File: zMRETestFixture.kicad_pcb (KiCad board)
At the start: 2 copper layers, 106.7 x 124.5 mm, 120 parts, among them J1 Conn_01x01, J2 Conn_01x01, J3 Conn_01x01_Female, J4 Conn_01x01_Female, J5 Conn_01x01, J6 Conn_01x01, J7 Conn_01x01, J8 Conn_01x01, J9 Conn_02x05_Counter_Clockwise, SW1 SW_Push, SW2 SW_Push, U1 molex_48pin_MRE

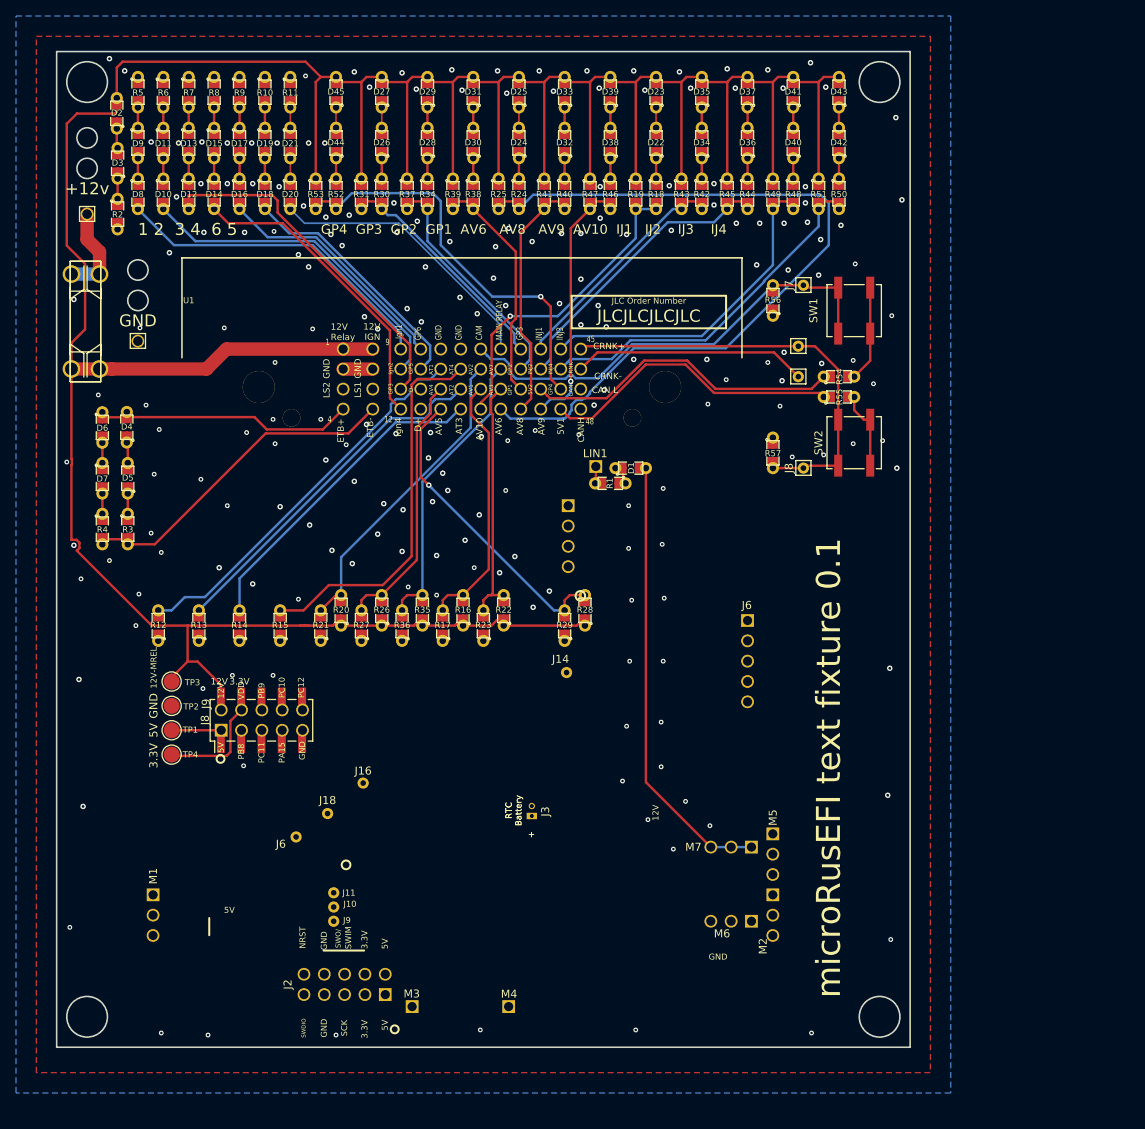
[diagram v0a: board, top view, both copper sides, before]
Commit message: DRAFT`
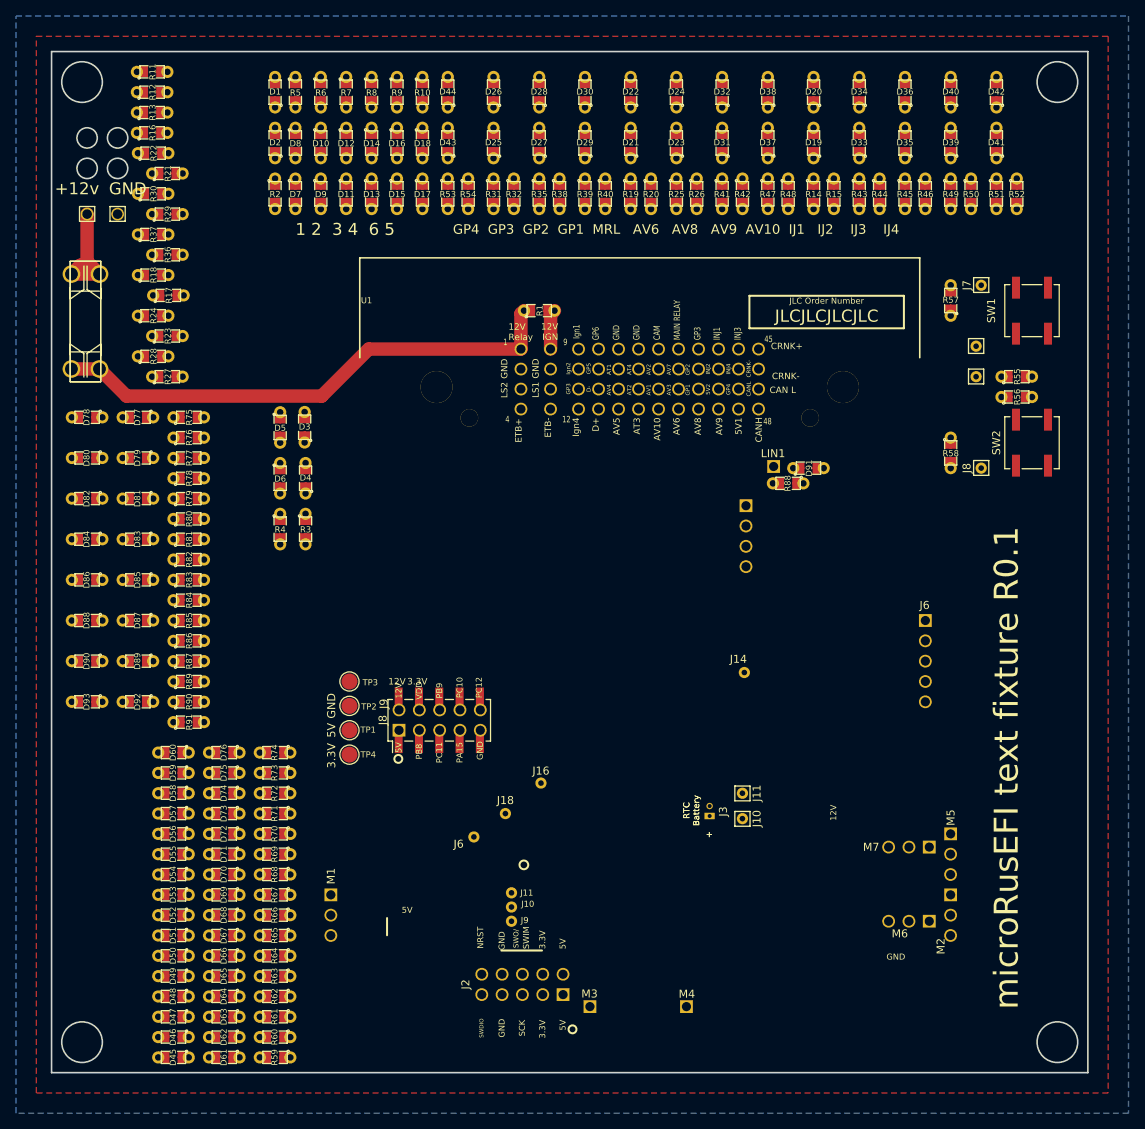
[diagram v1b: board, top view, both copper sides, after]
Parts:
- removed R34: 1k, rusefi_lib:SM0805_jumper
- added D46: 1N4148WS, rusefi_lib:SM0805_jumper, F.Cu at (45.1, 150.5)
- added D47: 1N4148WS, rusefi_lib:SM0805_jumper, F.Cu at (45.1, 148.0)
- added D48: 1N4148WS, rusefi_lib:SM0805_jumper, F.Cu at (45.1, 145.4)
- added D49: 1N4148WS, rusefi_lib:SM0805_jumper, F.Cu at (45.1, 142.9)
- added D50: 1N4148WS, rusefi_lib:SM0805_jumper, F.Cu at (45.1, 140.3)
- added D51: 1N4148WS, rusefi_lib:SM0805_jumper, F.Cu at (45.1, 137.8)
- added D52: 1N4148WS, rusefi_lib:SM0805_jumper, F.Cu at (45.1, 135.3)
- added D53: 1N4148WS, rusefi_lib:SM0805_jumper, F.Cu at (45.1, 132.7)
- added D54: 1N4148WS, rusefi_lib:SM0805_jumper, F.Cu at (45.1, 130.2)
- added D55: 1N4148WS, rusefi_lib:SM0805_jumper, F.Cu at (45.1, 127.6)
- added D56: 1N4148WS, rusefi_lib:SM0805_jumper, F.Cu at (45.1, 125.1)
- added D57: 1N4148WS, rusefi_lib:SM0805_jumper, F.Cu at (45.1, 122.6)
- added D58: 1N4148WS, rusefi_lib:SM0805_jumper, F.Cu at (45.1, 120.0)
- added D59: 1N4148WS, rusefi_lib:SM0805_jumper, F.Cu at (45.1, 117.5)
- added D60: 1N4148WS, rusefi_lib:SM0805_jumper, F.Cu at (45.1, 114.9)
- added D61: GRN, rusefi_lib:SM0805_jumper, F.Cu at (51.4, 153.0)
- added D62: GRN, rusefi_lib:SM0805_jumper, F.Cu at (51.4, 150.5)
- added D63: GRN, rusefi_lib:SM0805_jumper, F.Cu at (51.4, 148.0)
- added D64: GRN, rusefi_lib:SM0805_jumper, F.Cu at (51.4, 145.4)
- added D65: GRN, rusefi_lib:SM0805_jumper, F.Cu at (51.4, 142.9)
- added D66: GRN, rusefi_lib:SM0805_jumper, F.Cu at (51.4, 140.3)
- added D67: GRN, rusefi_lib:SM0805_jumper, F.Cu at (51.4, 137.8)
- added D68: GRN, rusefi_lib:SM0805_jumper, F.Cu at (51.4, 135.3)
- added D69: GRN, rusefi_lib:SM0805_jumper, F.Cu at (51.4, 132.7)
- added D70: GRN, rusefi_lib:SM0805_jumper, F.Cu at (51.4, 130.2)
- added D71: GRN, rusefi_lib:SM0805_jumper, F.Cu at (51.4, 127.6)
- added D72: GRN, rusefi_lib:SM0805_jumper, F.Cu at (51.4, 125.1)
- added D73: GRN, rusefi_lib:SM0805_jumper, F.Cu at (51.4, 122.6)
- added D74: GRN, rusefi_lib:SM0805_jumper, F.Cu at (51.4, 120.0)
- added D75: GRN, rusefi_lib:SM0805_jumper, F.Cu at (51.4, 117.5)
- added D76: GRN, rusefi_lib:SM0805_jumper, F.Cu at (51.4, 114.9)
- added D77: RED, rusefi_lib:SM0805_jumper, F.Cu at (40.6, 73.0)
- added D78: 1N4148WS, rusefi_lib:SM0805_jumper, F.Cu at (34.3, 73.0)
- added D79: RED, rusefi_lib:SM0805_jumper, F.Cu at (40.6, 78.1)
- added D80: 1N4148WS, rusefi_lib:SM0805_jumper, F.Cu at (34.3, 78.1)
- added D81: RED, rusefi_lib:SM0805_jumper, F.Cu at (40.6, 83.2)
- added D82: 1N4148WS, rusefi_lib:SM0805_jumper, F.Cu at (34.3, 83.2)
- added D83: RED, rusefi_lib:SM0805_jumper, F.Cu at (40.6, 88.3)
- added D84: 1N4148WS, rusefi_lib:SM0805_jumper, F.Cu at (34.3, 88.3)
- added D85: RED, rusefi_lib:SM0805_jumper, F.Cu at (40.6, 93.3)
- added D86: 1N4148WS, rusefi_lib:SM0805_jumper, F.Cu at (34.3, 93.3)
- added D87: RED, rusefi_lib:SM0805_jumper, F.Cu at (40.6, 98.4)
- added D88: 1N4148WS, rusefi_lib:SM0805_jumper, F.Cu at (34.3, 98.4)
- added D89: RED, rusefi_lib:SM0805_jumper, F.Cu at (40.6, 103.5)
- added D90: 1N4148WS, rusefi_lib:SM0805_jumper, F.Cu at (34.3, 103.5)
- added D91: 1N4148WS, rusefi_lib:SM0805_jumper, F.Cu at (124.5, 79.4)
- added D92: RED, rusefi_lib:SM0805_jumper, F.Cu at (40.6, 108.6)
- added D93: 1N4148WS, rusefi_lib:SM0805_jumper, F.Cu at (34.3, 108.6)
- added J10: Conn_01x01, Connector_Pin:Pin_D0.7mm_L6.5mm_W1.8mm_FlatFork, F.Cu at (116.2, 123.2)
- added J11: Conn_01x01, Connector_Pin:Pin_D0.7mm_L6.5mm_W1.8mm_FlatFork, F.Cu at (116.2, 120.0)
- added R32: 5k, rusefi_lib:SM0805_jumper, F.Cu at (87.6, 45.1)
- added R58: 470k, rusefi_lib:SM0805_jumper, F.Cu at (142.2, 77.5)
- added R59: 1k, rusefi_lib:SM0805_jumper, F.Cu at (57.8, 153.0)
- added R60: 1k, rusefi_lib:SM0805_jumper, F.Cu at (57.8, 150.5)
- added R61: 1k, rusefi_lib:SM0805_jumper, F.Cu at (57.8, 148.0)
- added R62: 1k, rusefi_lib:SM0805_jumper, F.Cu at (57.8, 145.4)
- added R63: 1k, rusefi_lib:SM0805_jumper, F.Cu at (57.8, 142.9)
- added R64: 1k, rusefi_lib:SM0805_jumper, F.Cu at (57.8, 140.3)
- added R65: 1k, rusefi_lib:SM0805_jumper, F.Cu at (57.8, 137.8)
- added R66: 1k, rusefi_lib:SM0805_jumper, F.Cu at (57.8, 135.3)
- added R67: 1k, rusefi_lib:SM0805_jumper, F.Cu at (57.8, 132.7)
- added R68: 1k, rusefi_lib:SM0805_jumper, F.Cu at (57.8, 130.2)
- added R69: 1k, rusefi_lib:SM0805_jumper, F.Cu at (57.8, 127.6)
- added R70: 1k, rusefi_lib:SM0805_jumper, F.Cu at (57.8, 125.1)
- added R71: 1k, rusefi_lib:SM0805_jumper, F.Cu at (57.8, 122.6)
- added R72: 1k, rusefi_lib:SM0805_jumper, F.Cu at (57.8, 120.0)
- added R73: 1k, rusefi_lib:SM0805_jumper, F.Cu at (57.8, 117.5)
- added R74: 1k, rusefi_lib:SM0805_jumper, F.Cu at (57.8, 114.9)
- added R75: 1k, rusefi_lib:SM0805_jumper, F.Cu at (47.0, 73.0)
- added R76: 5k, rusefi_lib:SM0805_jumper, F.Cu at (47.0, 75.6)
- added R77: 1k, rusefi_lib:SM0805_jumper, F.Cu at (47.0, 78.1)
- added R78: 5k, rusefi_lib:SM0805_jumper, F.Cu at (47.0, 80.6)
- added R79: 1k, rusefi_lib:SM0805_jumper, F.Cu at (47.0, 83.2)
- added R80: 5k, rusefi_lib:SM0805_jumper, F.Cu at (47.0, 85.7)
- added R81: 1k, rusefi_lib:SM0805_jumper, F.Cu at (47.0, 88.3)
- added R82: 5k, rusefi_lib:SM0805_jumper, F.Cu at (47.0, 90.8)
- added R83: 1k, rusefi_lib:SM0805_jumper, F.Cu at (47.0, 93.3)
- added R84: 5k, rusefi_lib:SM0805_jumper, F.Cu at (47.0, 95.9)
- added R85: 1k, rusefi_lib:SM0805_jumper, F.Cu at (47.0, 98.4)
- added R86: 5k, rusefi_lib:SM0805_jumper, F.Cu at (47.0, 101.0)
- added R87: 1k, rusefi_lib:SM0805_jumper, F.Cu at (47.0, 103.5)
- added R88: 1k, rusefi_lib:SM0805_jumper, F.Cu at (121.9, 81.3)
- added R89: 5k, rusefi_lib:SM0805_jumper, F.Cu at (47.0, 106.0)
- added R90: 1k, rusefi_lib:SM0805_jumper, F.Cu at (47.0, 108.6)
- added R91: 5k, rusefi_lib:SM0805_jumper, F.Cu at (47.0, 111.1)
- D10, D12, D14, D16, D18, D8: value 1N4148WS -> BLU
- D11, D13, D15, D17, D9: value BLU -> 1N4148WS
- D19: value BLU -> RED
- D2: value 1N4148WS -> GRN
- D21: value GRN -> RED
- D22, D24, D26, D28, D30, D32, D34, D36, D38, D40, D42, D44: value RED -> 1N4148WS
- D23, D25, D27, D29, D31, D33, D35, D37, D39, D41, D43: value 1N4148WS -> RED
- D3: value GRN -> 1N4148WS
- D4: value 1N4148WS -> YEL(593NM)
- D5: value YEL(593NM) -> 1N4148WS
- D6: value 1N4148WS -> YEL(570NM)
- D7: value YEL(570NM) -> 1N4148WS
- R1: value 1k -> 0R
- R12, R24, R30: value 1k -> 2k2
- R13: value 2k2 -> 3k3
- R14: value 3k3 -> 1k
- R15: value 4k7 -> 5k
- R16: value 10k -> 4k7
- R17: value 220R -> 10k
- R19, R25, R31, R35, R39, R41, R43, R45, R47, R49, R51, R53: value 5k -> 1k
- R21: value 220R -> 5k
- R22: value 10k -> 1k
- R23, R27: value 470R -> 10k
- R28: value 10k -> 3k3
- R29, R36, R38, R40, R42, R44, R46, R48, R50, R52: value 1k -> 5k
- R37: value 5k -> 4k7
- R56: value 470k -> 5k
- moved D45 122.3 mm to (45.1, 153.0), turned to 180 degrees
- moved R14 89.8 mm to (125.1, 45.1), turned to 270 degrees
- moved R15 87.8 mm to (127.6, 45.1), turned to 270 degrees
- moved R52 85.1 mm to (150.5, 45.1)
- moved R22 72.0 mm to (42.5, 40.0), turned to 0 degrees
- moved R29 71.5 mm to (44.3, 47.6), turned to 0 degrees
- moved R16 71.2 mm to (42.4, 37.5), turned to 0 degrees
- moved D19 68.6 mm to (125.1, 38.7), turned to 90 degrees
- moved R12 66.7 mm to (42.4, 32.4), turned to 0 degrees
- moved D20 66.6 mm to (125.1, 32.4), turned to 90 degrees
- moved R26 65.3 mm to (110.5, 45.1), turned to 270 degrees
- moved R20 64.9 mm to (104.8, 45.1), turned to 270 degrees
- moved D1 64.7 mm to (57.8, 32.4), turned to 90 degrees
- moved R13 64.4 mm to (42.4, 34.9), turned to 0 degrees
- moved R18 63.7 mm to (42.5, 55.2), turned to 0 degrees
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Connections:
- D1 pad 2: /12V_SAFE -> /12V_MREL
- D10 pad 2: /Ign2 -> Net-(D10-Pad2)
- D11 pad 2: Net-(D10-Pad1) -> /Ign3
- D12 pad 2: /Ign3 -> Net-(D11-Pad1)
- D13 pad 2: Net-(D12-Pad1) -> /Ign4
- D14 pad 2: /Ign4 -> Net-(D13-Pad1)
- D15 pad 2: Net-(D14-Pad1) -> /GP6
- D16 pad 2: /GP6 -> Net-(D15-Pad1)
- D17 pad 2: Net-(D16-Pad1) -> /GP5
- D18 pad 2: /GP5 -> Net-(D17-Pad1)
- D19 pad 2: Net-(D18-Pad1) -> Net-(D19-Pad2)
- D2 pad 2: /12V_KEY -> Net-(D1-Pad1)
- D20 pad 1: Net-(D20-Pad1) -> Net-(D19-Pad2)
- D20 pad 2: /MAIN_RELAY -> /12V_MREL
- D21 pad 2: Net-(D20-Pad1) -> Net-(D21-Pad2)
- D22 pad 1: Net-(D22-Pad1) -> Net-(D21-Pad2)
- D22 pad 2: Net-(D22-Pad2) -> /12V_MREL
- D23 pad 1: Net-(D22-Pad2) -> Net-(D23-Pad1)
- D23 pad 2: /12V_KEY -> Net-(D23-Pad2)
- D24 pad 1: Net-(D24-Pad1) -> Net-(D23-Pad2)
- D24 pad 2: Net-(D24-Pad2) -> /12V_MREL
- D25 pad 1: Net-(D24-Pad2) -> Net-(D25-Pad1)
- D25 pad 2: /12V_KEY -> Net-(D25-Pad2)
- D26 pad 1: Net-(D26-Pad1) -> Net-(D25-Pad2)
- D26 pad 2: Net-(D26-Pad2) -> /12V_MREL
- D27 pad 1: Net-(D26-Pad2) -> Net-(D27-Pad1)
- D27 pad 2: /12V_KEY -> Net-(D27-Pad2)
- D28 pad 1: Net-(D28-Pad1) -> Net-(D27-Pad2)
- D28 pad 2: Net-(D28-Pad2) -> /12V_MREL
- D29 pad 1: Net-(D28-Pad2) -> Net-(D29-Pad1)
- D29 pad 2: /12V_KEY -> Net-(D29-Pad2)
- D3 pad 2: Net-(D2-Pad1) -> /E-THROTTLE+
- D30 pad 1: Net-(D30-Pad1) -> Net-(D29-Pad2)
- D30 pad 2: Net-(D30-Pad2) -> /12V_MREL
- D31 pad 1: Net-(D30-Pad2) -> Net-(D31-Pad1)
- D31 pad 2: /12V_KEY -> Net-(D31-Pad2)
- D32 pad 1: Net-(D32-Pad1) -> Net-(D31-Pad2)
- D32 pad 2: Net-(D32-Pad2) -> /12V_MREL
- D33 pad 1: Net-(D32-Pad2) -> Net-(D33-Pad1)
- D33 pad 2: /12V_KEY -> Net-(D33-Pad2)
- D34 pad 1: Net-(D34-Pad1) -> Net-(D33-Pad2)
- D34 pad 2: Net-(D34-Pad2) -> /12V_MREL
- D35 pad 1: Net-(D34-Pad2) -> Net-(D35-Pad1)
- D35 pad 2: /12V_KEY -> Net-(D35-Pad2)
- D36 pad 1: Net-(D36-Pad1) -> Net-(D35-Pad2)
- D36 pad 2: Net-(D36-Pad2) -> /12V_MREL
- D37 pad 1: Net-(D36-Pad2) -> Net-(D37-Pad1)
- D37 pad 2: /12V_KEY -> Net-(D37-Pad2)
- D38 pad 1: Net-(D38-Pad1) -> Net-(D37-Pad2)
- D38 pad 2: Net-(D38-Pad2) -> /12V_MREL
- D39 pad 1: Net-(D38-Pad2) -> Net-(D39-Pad1)
- D39 pad 2: /12V_KEY -> Net-(D39-Pad2)
- D4 pad 2: /E-THROTTLE+ -> Net-(D3-Pad1)
- D40 pad 1: Net-(D40-Pad1) -> Net-(D39-Pad2)
- D40 pad 2: Net-(D40-Pad2) -> /12V_MREL
- D41 pad 1: Net-(D40-Pad2) -> Net-(D41-Pad1)
- D41 pad 2: /12V_KEY -> Net-(D41-Pad2)
- D42 pad 1: Net-(D42-Pad1) -> Net-(D41-Pad2)
- D42 pad 2: Net-(D42-Pad2) -> /12V_MREL
- D43 pad 1: Net-(D42-Pad2) -> Net-(D43-Pad1)
- D43 pad 2: /12V_KEY -> Net-(D43-Pad2)
- D44 pad 1: Net-(D44-Pad1) -> Net-(D43-Pad2)
- D44 pad 2: Net-(D44-Pad2) -> /12V_MREL
- D45 pad 1: Net-(D44-Pad2) -> Net-(D45-Pad1)
- D45 pad 2: /12V_KEY -> /PA15
- D5 pad 1: Net-(D5-Pad1) -> /E-THROTTLE+
- D5 pad 2: Net-(D4-Pad1) -> Net-(D5-Pad2)
- D6 pad 1: /E-THROTTLE+ -> Net-(D5-Pad2)
- D7 pad 1: Net-(D6-Pad2) -> Net-(D7-Pad1)
- D7 pad 2: Net-(D7-Pad2) -> /Ign1
- D8 pad 2: /Ign1 -> Net-(D7-Pad1)
- D9 pad 1: Net-(D9-Pad1) -> Net-(D10-Pad2)
- D9 pad 2: Net-(D8-Pad1) -> /Ign2
- J4 pad 1: /12V_KEY -> /12V_MREL
- J9 pad 2: /12V_KEY -> /12V_MREL
- R1 pad 1: Net-(D1-Pad1) -> /12V_MREL
- R1 pad 2: /LINBUS -> /12V_KEY
- R10 pad 2: Net-(D19-Pad1) -> Net-(D18-Pad1)
- R11 pad 2: Net-(D21-Pad1) -> /AT1
- R12 pad 2: /AT1 -> /AT2
- R13 pad 2: /AT2 -> /AT3
- R14 pad 1: GND -> Net-(D19-Pad1)
- R14 pad 2: /AT3 -> /AV10
- R15 pad 1: GND -> /12V_MREL
- R15 pad 2: /AT4 -> /AV10
- R16 pad 1: /12V_KEY -> GND
- R16 pad 2: /AV1 -> /AT4
- R17 pad 1: GND -> /5V1
- R18 pad 1: Net-(D22-Pad1) -> GND
- R18 pad 2: /AV10 -> /AV1
- R19 pad 1: /12V_KEY -> Net-(D21-Pad1)
- R19 pad 2: /AV10 -> /MAIN_RELAY
- R2 pad 1: Net-(D3-Pad1) -> Net-(D2-Pad1)
- R20 pad 1: /12V_KEY -> /12V_MREL
- R20 pad 2: /AV2 -> /MAIN_RELAY
- R21 pad 1: GND -> /5V1
- R22 pad 1: /12V_KEY -> GND
- R22 pad 2: /AV3 -> /AV2
- R23 pad 1: GND -> /5V1
- R24 pad 1: Net-(D24-Pad1) -> GND
- R24 pad 2: /AV6 -> /AV3
- R25 pad 1: /12V_KEY -> Net-(D23-Pad1)
- R26 pad 1: /12V_KEY -> /12V_MREL
- R26 pad 2: /AV4 -> /AV6
- R27 pad 1: GND -> /5V1
- R28 pad 1: /12V_KEY -> GND
- R28 pad 2: /AV5 -> /AV4
- R29 pad 1: GND -> /5V2
- R3 pad 1: Net-(D5-Pad1) -> Net-(D4-Pad1)
- R30 pad 1: Net-(D26-Pad1) -> GND
- R30 pad 2: /GP3 -> /AV5
- R31 pad 1: /12V_KEY -> Net-(D25-Pad1)
- R35 pad 1: /12V_KEY -> Net-(D27-Pad1)
- R35 pad 2: /AV7 -> /GP2
- R36 pad 1: GND -> /5V2
- R37 pad 1: /12V_KEY -> GND
- R37 pad 2: /GP2 -> /AV7
- R38 pad 1: Net-(D30-Pad1) -> /12V_MREL
- R38 pad 2: /GP1 -> /GP2
- R39 pad 1: /12V_KEY -> Net-(D29-Pad1)
- R4 pad 1: Net-(D7-Pad2) -> Net-(D6-Pad2)
- R40 pad 1: Net-(D32-Pad1) -> /12V_MREL
- R40 pad 2: /AV8 -> /GP1
- R41 pad 1: /12V_KEY -> Net-(D31-Pad1)
- R42 pad 1: Net-(D34-Pad1) -> /12V_MREL
- R42 pad 2: /INJECTOR-1 -> /AV8
- R43 pad 1: /12V_KEY -> Net-(D33-Pad1)
- R44 pad 1: Net-(D36-Pad1) -> /12V_MREL
- R44 pad 2: /INJECTOR-2 -> /INJECTOR-1
- R45 pad 1: /12V_KEY -> Net-(D35-Pad1)
- R46 pad 1: Net-(D38-Pad1) -> /12V_MREL
- R46 pad 2: /AV9 -> /INJECTOR-2
- R47 pad 1: /12V_KEY -> Net-(D37-Pad1)
- R48 pad 1: Net-(D40-Pad1) -> /12V_MREL
- R48 pad 2: /INJECTOR-3 -> /AV9
- R49 pad 1: /12V_KEY -> Net-(D39-Pad1)
- R5 pad 2: Net-(D9-Pad1) -> Net-(D8-Pad1)
- R50 pad 1: Net-(D42-Pad1) -> /12V_MREL
- R50 pad 2: /INJECTOR-4 -> /INJECTOR-3
- R51 pad 1: /12V_KEY -> Net-(D41-Pad1)
- R52 pad 1: Net-(D44-Pad1) -> /12V_MREL
- R52 pad 2: /GP4 -> /INJECTOR-4
- R53 pad 1: /12V_KEY -> Net-(D43-Pad1)
- R54 pad 1: /5V2 -> /12V_MREL
- R54 pad 2: Net-(R54-Pad2) -> /GP4
- R55 pad 1: /5V1 -> /5V2
- R56 pad 1: GND -> /5V1
- R56 pad 2: /CAM_SENSOR -> Net-(R56-Pad2)
- R57 pad 2: /CRNK+ -> /CAM_SENSOR
- R6 pad 2: Net-(D11-Pad1) -> Net-(D10-Pad1)
- R7 pad 2: Net-(D13-Pad1) -> Net-(D12-Pad1)
- R8 pad 2: Net-(D15-Pad1) -> Net-(D14-Pad1)
- R9 pad 2: Net-(D17-Pad1) -> Net-(D16-Pad1)
- SW1 pad 1: Net-(R54-Pad2) -> Net-(R55-Pad2)
- SW2 pad 1: Net-(R55-Pad2) -> Net-(R56-Pad2)
- TP3 pad 1: /12V_KEY -> /12V_MREL
- U1 pad 1: /12V_KEY -> /12V_MREL
- U1 pad 3: (no net) -> /LS2
- U1 pad 7: (no net) -> /LS1
- U1 pad J10: (no net) -> /PE6
- U1 pad J11: (no net) -> /PE5
- U1 pad J14: (no net) -> /OUT_7
- U1 pad J16: (no net) -> /PD0
- U1 pad J18: (no net) -> /PB7
- U1 pad J203: (no net) -> GND
- U1 pad J204: (no net) -> GND
- U1 pad J207: (no net) -> /VDD
- U1 pad J208: (no net) -> /VDD
- U1 pad J209: (no net) -> /5V
- U1 pad J210: (no net) -> /5V
- U1 pad J31: (no net) -> GND
- U1 pad J32: (no net) -> /Vrtc
- U1 pad J51: (no net) -> /IGN_OUT_1
- U1 pad J52: (no net) -> /IGN_OUT_2
- U1 pad J53: (no net) -> /IGN_OUT_3
- U1 pad J54: (no net) -> /IGN_OUT_4
- U1 pad J6: (no net) -> /PE0
- U1 pad J61: (no net) -> /OUT_14
- U1 pad J62: (no net) -> /OUT_15
- U1 pad J63: (no net) -> /OUT_16
- U1 pad J64: (no net) -> /OUT_17
- U1 pad J65: (no net) -> /OUT_18
- U1 pad J802: /12V_KEY -> /12V_MREL
- U1 pad J9: (no net) -> /PC13
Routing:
- net /12V_KEY: track 464.6 -> 5.01 mm
- net /AV6: track 101.0 -> 0.00 mm
- net /12V_MREL: track 0.00 -> 65.0 mm
- net /CAM_SENSOR: track 58.7 -> 0.00 mm
- net /12V_SAFE: track 56.8 -> 0.00 mm
- net /CRNK+: track 54.8 -> 0.00 mm
- net /GP4: track 52.3 -> 0.00 mm, vias 1 -> 0
- net /AT1: track 49.8 -> 0.00 mm
- net /AT4: track 48.6 -> 0.00 mm
- net /INJECTOR-4: track 46.6 -> 0.00 mm
- net /AT2: track 45.8 -> 0.00 mm
- net /Ign3: track 44.0 -> 0.00 mm
- net /Ign2: track 42.9 -> 0.00 mm
- net /E-THROTTLE-: track 42.7 -> 0.00 mm
- net /INJECTOR-3: track 42.6 -> 0.00 mm
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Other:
- board size 106.7 x 124.5 mm -> 129.5 x 127.6 mm
- board text added: "GP4 GP3 GP2 GP1 MRL AV6 AV8 AV9 AV10 IJ1 IJ2 IJ3 IJ4"
- board text added: "microRusEFI text fixture R0.1"
- board text removed: "12V-MREL"
- board text removed: "GP4 GP3 GP2 GP1 AV6 AV8 AV9 AV10 IJ1 IJ2 IJ3 IJ4"
- board text removed: "microRusEFI text fixture 0.1"
